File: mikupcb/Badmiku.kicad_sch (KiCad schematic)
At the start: 8 parts, among them J1 Conn_01x04_Pin, J2 Conn_01x01_Pin, J3 Conn_01x08_Pin, SW1 SW_Push, SW2 SW_Push, SW3 SW_Push, U1 RP2040

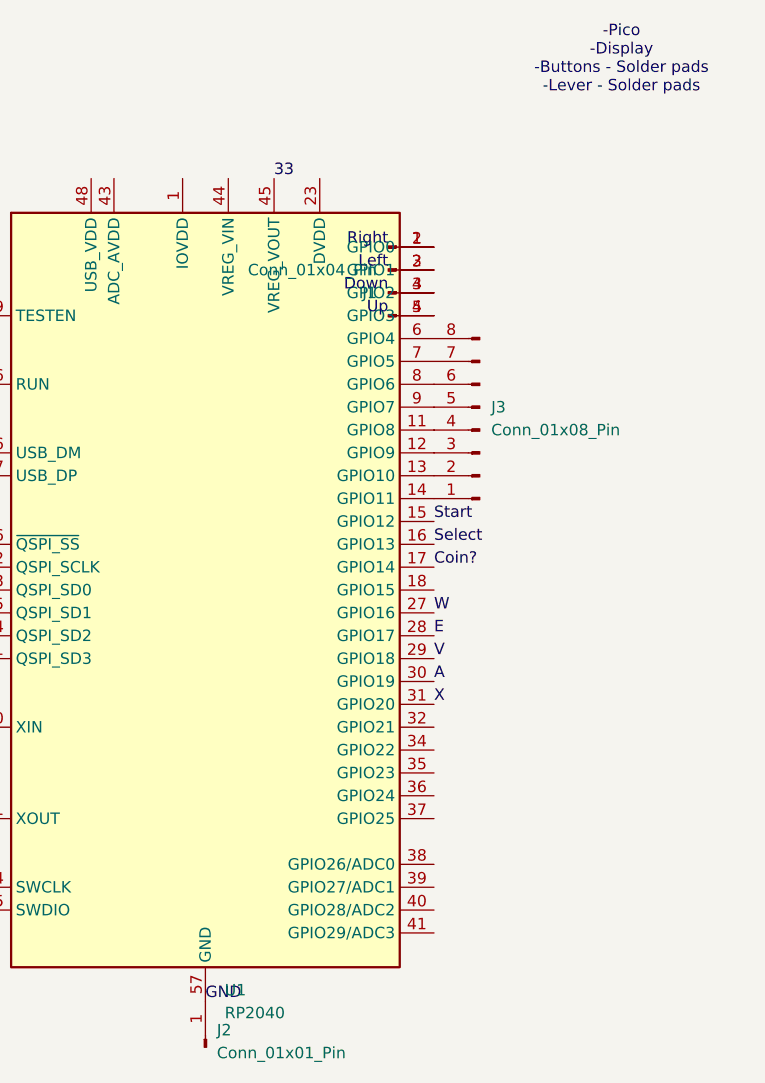
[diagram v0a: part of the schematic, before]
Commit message: Add files via upload
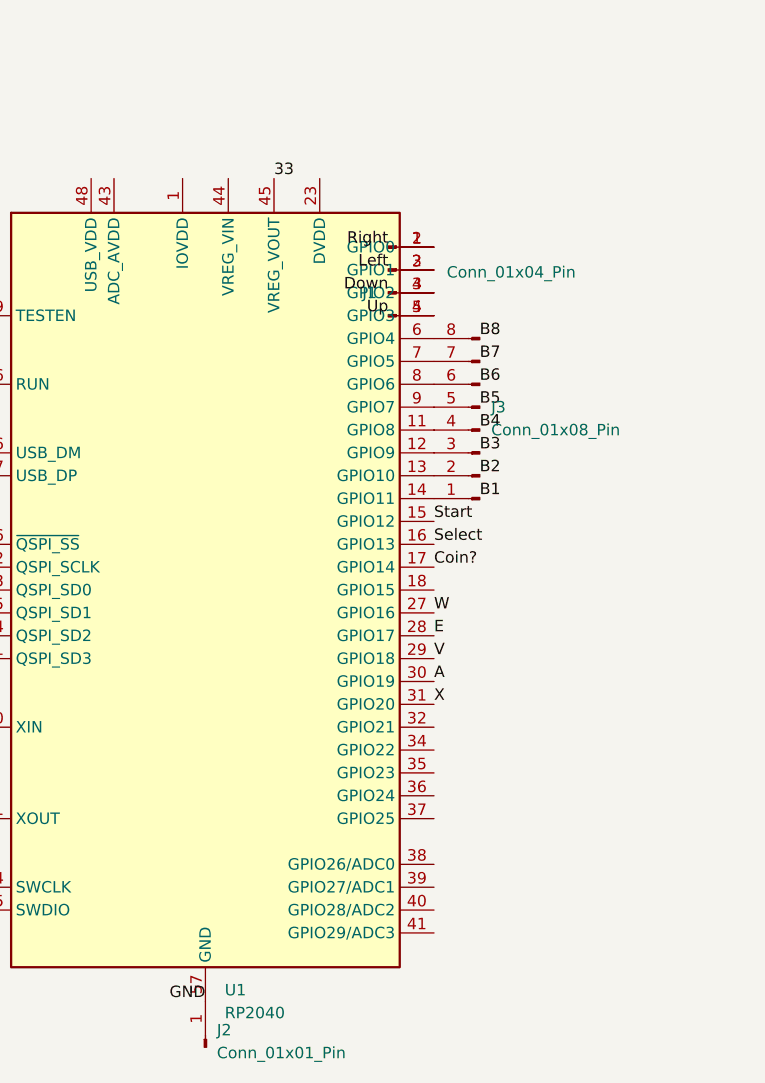
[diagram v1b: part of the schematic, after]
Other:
- note removed: "-Pico -Display -Buttons - Solder pads -Lever - Solder pads"
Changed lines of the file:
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@@
 	(generator_version "10.0")
 	(paper "A4")
-	(text "-Pico\n-Display\n-Buttons - Solder pads\n-Lever - Solder pads\n"
-		(exclude_from_sim no)
-		(at 249.428 22.352 0)
-		(effects
-			(font
-				(size 1.27 1.27)
-			)
-		)
-	)
 	(no_connect
 		(at 129.54 63.5)
@@
 		)
 	)
+	(label "B1"
+		(at 233.68 71.12 0)
+		(effects
+			(font
+				(size 1.27 1.27)
+			)
+			(justify left bottom)
+		)
+	)
 	(label "X"
 		(at 111.76 85.09 0)
@@
 		)
 	)
+	(label "B2"
+		(at 233.68 68.58 0)
+		(effects
+			(font
+				(size 1.27 1.27)
+			)
+			(justify left bottom)
+		)
+	)
 	(label "GND"
 		(at 87.63 105.41 0)
@@
 		)
 	)
+	(label "B3"
+		(at 233.68 66.04 0)
+		(effects
+			(font
+				(size 1.27 1.27)
+			)
+			(justify left bottom)
+		)
+	)
 	(label "Down"
 		(at 223.52 48.26 180)
@@
 		)
 	)
+	(label "B7"
+		(at 233.68 55.88 0)
+		(effects
+			(font
+				(size 1.27 1.27)
+			)
+			(justify left bottom)
+		)
+	)
 	(label "A"
 		(at 114.3 85.09 0)
@@
 		)
 	)
+	(label "B6"
+		(at 233.68 58.42 0)
+		(effects
+			(font
+				(size 1.27 1.27)
+			)
+			(justify left bottom)
+		)
+	)
 	(label "Start"
 		(at 92.71 105.41 0)
@@
 		)
 	)
+	(label "B5"
+		(at 233.68 60.96 0)
+		(effects
+			(font
+				(size 1.27 1.27)
+			)
+			(justify left bottom)
+		)
+	)
 	(label "GND"
-		(at 203.2 127 0)
-		(effects
-			(font
-				(size 1.27 1.27)
-			)
-			(justify left bottom)
+		(at 203.2 127 180)
+		(effects
+			(font
+				(size 1.27 1.27)
+			)
+			(justify right bottom)
 		)
 	)
@@
 		)
 	)
+	(label "B4"
+		(at 233.68 63.5 0)
+		(effects
+			(font
+				(size 1.27 1.27)
+			)
+			(justify left bottom)
+		)
+	)
 	(label "33"
 		(at 81.28 64.77 0)
@@
 	(label "E"
 		(at 127 85.09 0)
+		(effects
+			(font
+				(size 1.27 1.27)
+			)
+			(justify left bottom)
+		)
+	)
+	(label "B8"
+		(at 233.68 53.34 0)
 		(effects
 			(font
@@
 		(in_pos_files yes)
 		(dnp no)
-		(fields_autoplaced yes)
 		(property "Reference" "J1"
 			(at 222.25 48.2601 0)
@@
 		)
 		(property "Value" "Conn_01x04_Pin"
-			(at 222.25 45.7201 0)
-			(show_name no)
-			(do_not_autoplace no)
+			(at 244.348 45.974 0)
+			(show_name no)
+			(do_not_autoplace no)
